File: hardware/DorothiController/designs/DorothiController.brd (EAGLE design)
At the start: 101.6 x 50.8 mm, 25 parts

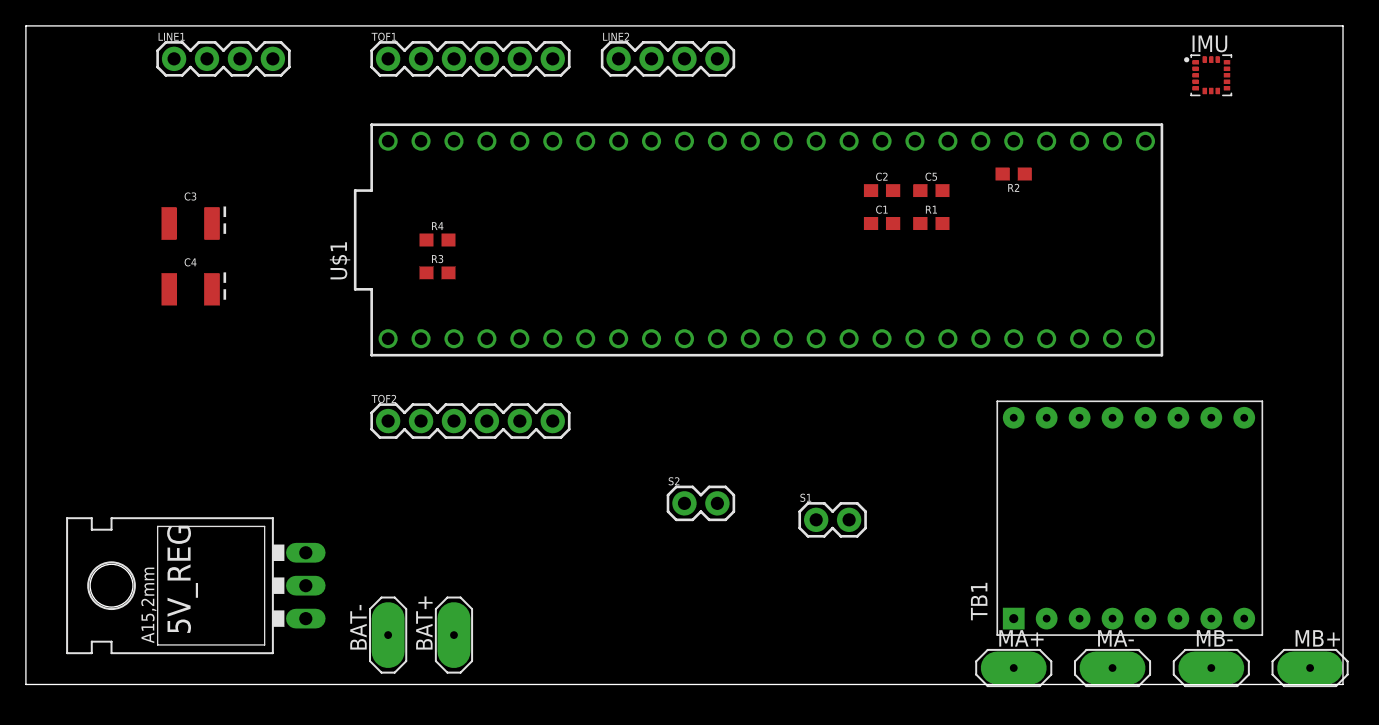
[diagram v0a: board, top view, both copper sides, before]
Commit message: controller ready
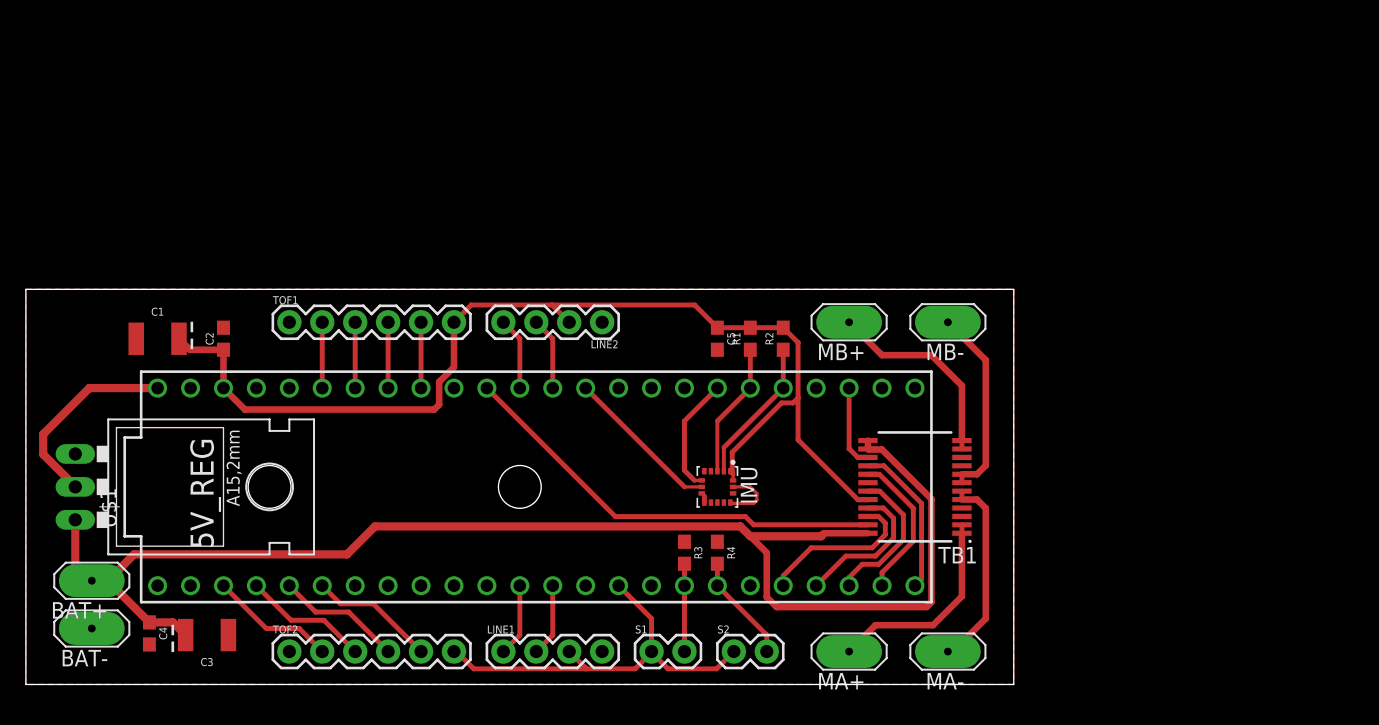
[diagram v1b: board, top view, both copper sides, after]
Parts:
- C1: value 0.1uF -> 10uF; device SparkFun-Capacitors:0603 -> SparkFun-Capacitors:EIA3528
- C4: value 10uF -> 0.1uF; device SparkFun-Capacitors:EIA3528 -> SparkFun-Capacitors:0603
- TB1: device TB6612FNG:TB6612FNG -> TB6612FNG:SOP65P760X160-24N
- moved C1 56.6 mm to (10.2, 26.7)
- moved LINE1 52.3 mm to (36.8, 2.54)
- moved C2 52.1 mm to (15.2, 26.7), turned to 90 degrees
- moved IMU 49.6 mm to (53.3, 15.2), turned to 270 degrees
- moved MB+ 44.5 mm to (63.5, 27.9), turned to 180 degrees
- moved MB- 33.5 mm to (71.1, 27.9), turned to 180 degrees
- moved R4 32.4 mm to (53.3, 10.2), turned to 270 degrees
- moved C3 31.8 mm to (14.0, 3.81), turned to 180 degrees
- moved R3 28.8 mm to (50.8, 10.2), turned to 270 degrees
- moved BAT+ 28.3 mm to (5.08, 8.00), turned to 180 degrees
- moved C4 26.7 mm to (9.53, 3.94), turned to 270 degrees
- moved U$1 26.1 mm to (38.1, 15.2)
- moved BAT- 22.9 mm to (5.08, 4.32), turned to 180 degrees
- moved R2 21.8 mm to (58.4, 26.7), turned to 90 degrees
- moved TOF1 21.7 mm to (20.3, 27.9)
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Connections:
- net N$6 renamed 5V_OUT
- net +12V: now also C3.A, C4.1, TB1.13, TB1.14, TB1.24; no longer C2.1, C4.A, TB1.VM
- net +3V3: now also C1.A, C2.1, LINE1.3, TB1.20; no longer C1.1, C3.A, LINE1.2, TB1.VCC
- net GND: now also C1.C, C4.2, LINE1.4, TB1.10, TB1.18, TB1.3, TB1.4, TB1.9; no longer C1.2, C4.C, LINE1.1, TB1.GND1, TB1.GND2, TB1.GND3
- net IMU_INT1: now also U$1.13; no longer U$1.35/A16
- net IMU_INT2: now also U$1.39/A20; no longer U$1.36/A17
- net LINE1_RS1: now also LINE1.1, U$1.10; no longer LINE1.3, U$1.12
- net LINE1_RS2: now also LINE1.2, U$1.11; no longer LINE1.4, U$1.13
- net MA+: now also TB1.1, TB1.2; no longer TB1.A1
- net MA-: now also TB1.5, TB1.6; no longer TB1.A2
- net MB+: now also TB1.11, TB1.12; no longer TB1.B1
- net MB-: now also TB1.7, TB1.8; no longer TB1.B2
- net M_AIN1: now also TB1.21, U$1.29; no longer TB1.AIN1, U$1.28
- net M_AIN2: now also TB1.22, U$1.28; no longer TB1.AIN2, U$1.29
- net M_BIN1: now also TB1.17, U$1.31/A12; no longer TB1.BIN1, U$1.30
- net M_BIN2: now also TB1.16, U$1.32/A13; no longer TB1.BIN2, U$1.31/A12
- net M_PWMA: now also TB1.23, U$1.16/A2; no longer TB1.PWMA, U$1.22/A8
- net M_PWMB: now also TB1.15, U$1.35/A16; no longer TB1.PWMB, U$1.23/A9
- net M_STBY: now also TB1.19, U$1.30; no longer TB1.STBY, U$1.32/A13
- net TOF1_READY: now also U$1.20/A6; no longer U$1.17/A3
- net TOF1_SHDN: now also U$1.21/A7; no longer U$1.20/A6
- net TOF2_SHDN: now also U$1.1; no longer U$1.5
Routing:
- net +3V3: track 0.00 -> 117.0 mm
- net +12V: track 0.00 -> 108.5 mm
- net M_PWMA: track 0.00 -> 33.8 mm
- net MA+: track 0.00 -> 16.0 mm
- net MB+: track 0.00 -> 15.6 mm
- net 5V_OUT: track 0.00 -> 15.4 mm
- net MA-: track 0.00 -> 15.2 mm
- net MB-: track 0.00 -> 15.0 mm
- net M_AIN2: track 0.00 -> 12.4 mm
- net IMU_INT1: track 0.00 -> 12.1 mm
- net M_BIN2: track 0.00 -> 11.9 mm
- net M_BIN1: track 0.00 -> 11.6 mm
- net M_STBY: track 0.00 -> 11.4 mm
- net M_AIN1: track 0.00 -> 11.3 mm
- net IMU_SCL: track 0.00 -> 11.3 mm
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- added copper zone on layer 1, net GND
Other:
- board size 101.6 x 50.8 mm -> 76.2 x 30.5 mm
